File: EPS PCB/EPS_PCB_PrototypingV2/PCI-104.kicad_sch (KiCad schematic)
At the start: 6 parts, among them J1 Conn_02x26_Row_Letter_First, J2 Conn_02x26_Row_Letter_First

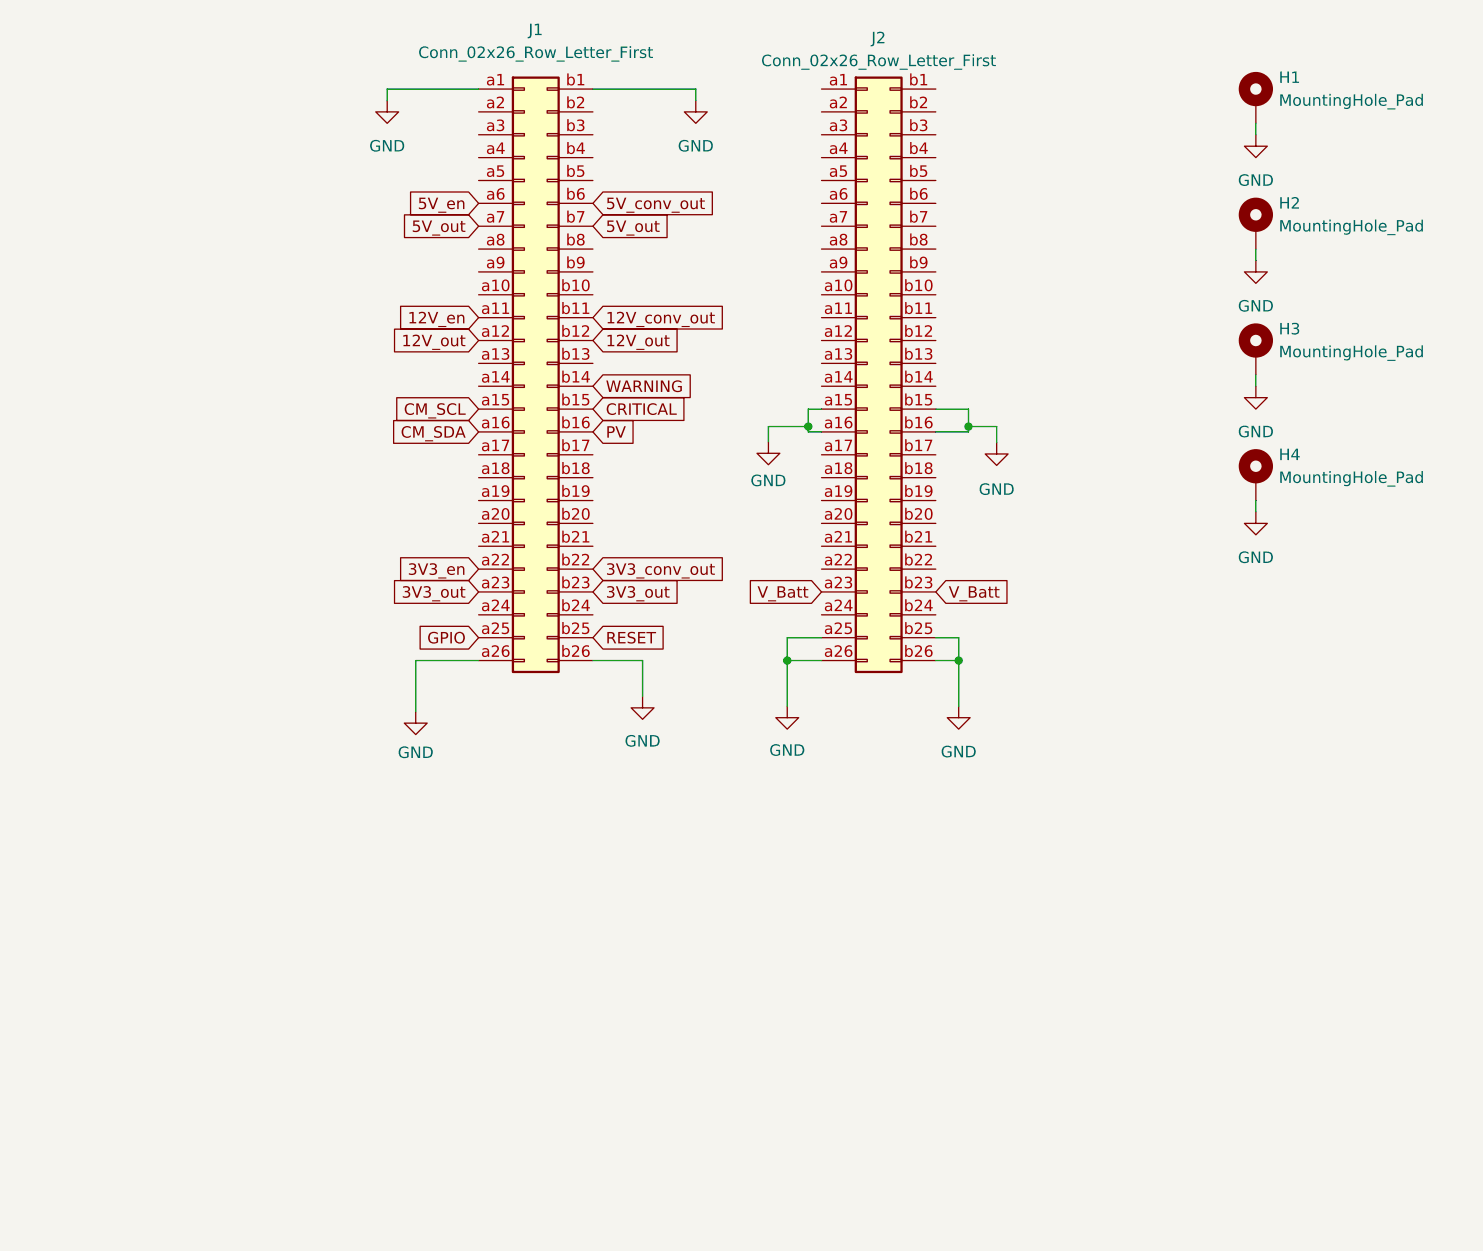
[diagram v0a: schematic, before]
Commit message: EPS PCB Ready for Order
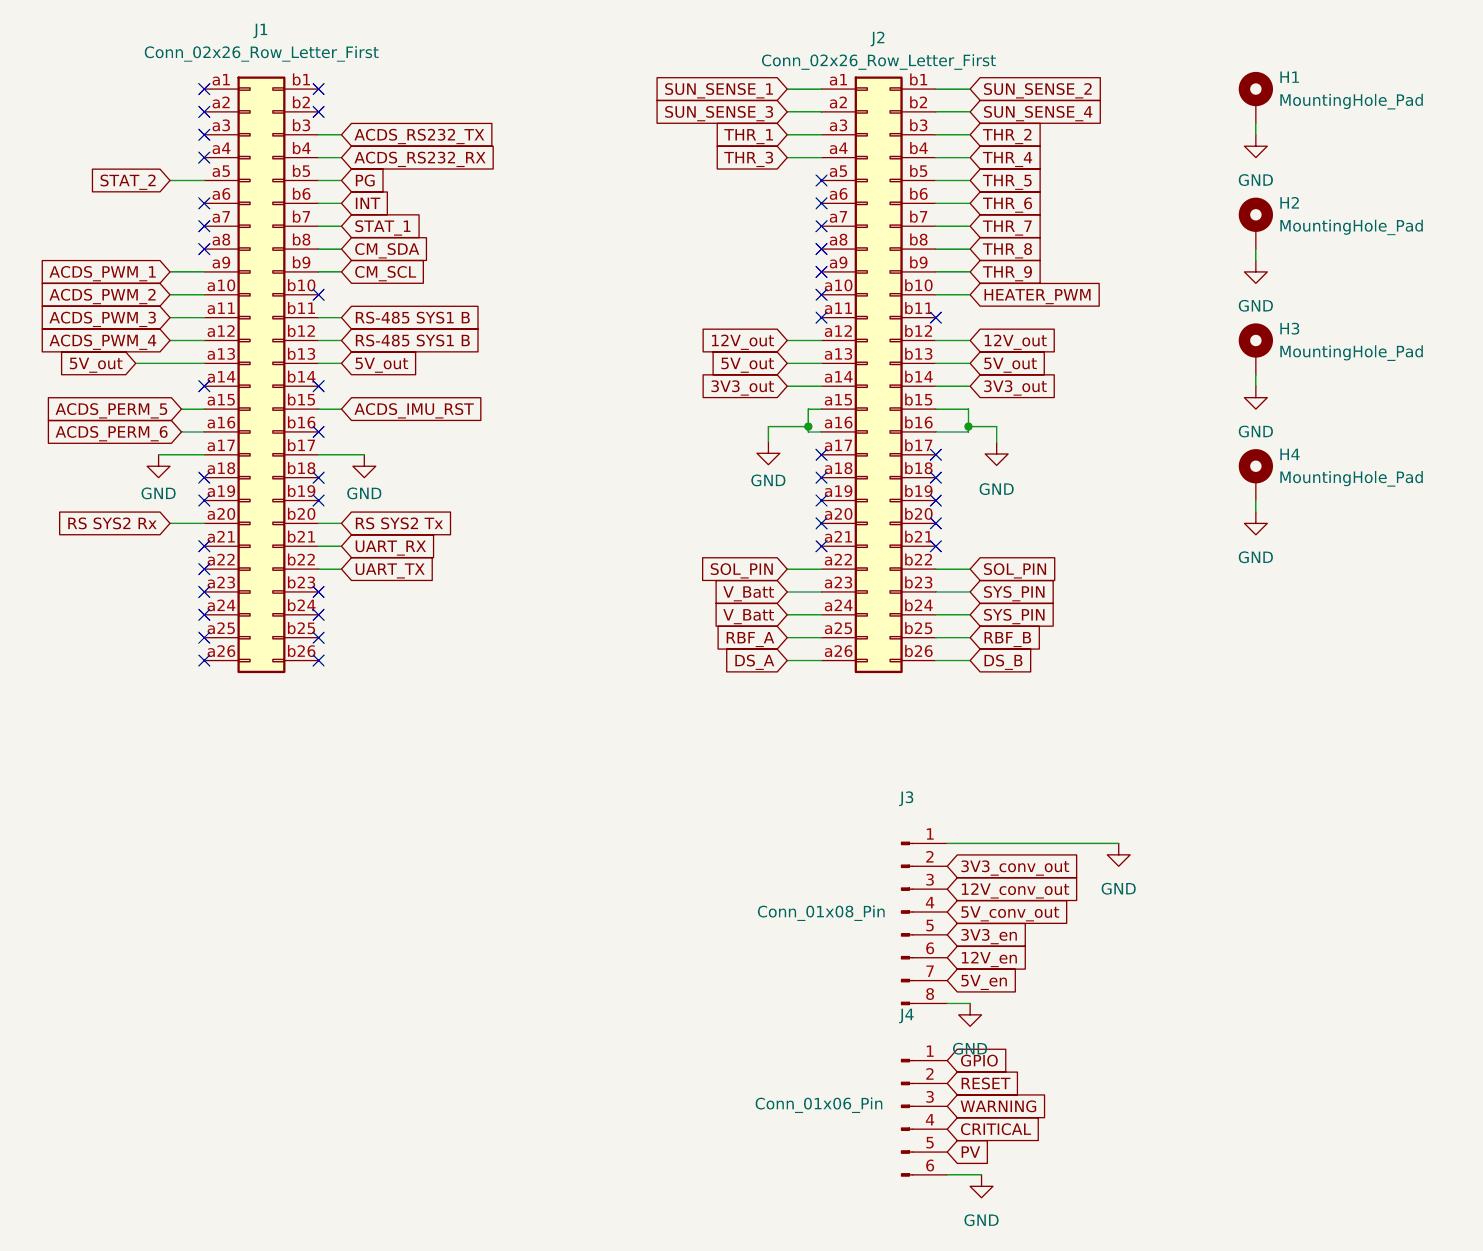
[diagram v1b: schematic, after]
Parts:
- added J3: Conn_01x08_Pin, Connector_PinHeader_2.54mm:PinHeader_1x08_P2.54mm_Vertical, symbol Connector:Conn_01x08_Pin
- added J4: Conn_01x06_Pin, Connector_PinHeader_2.54mm:PinHeader_1x06_P2.54mm_Horizontal, symbol Connector:Conn_01x06_Pin
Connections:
- net 12V_conv_out: now also J3.3 (Pin_3); no longer J1.b11 (Pin_b11)
- net 12V_en: now also J3.6 (Pin_6); no longer J1.a11 (Pin_a11)
- net 12V_out: now also J2.a12 (Pin_a12), J2.b12 (Pin_b12); no longer J1.a12 (Pin_a12), J1.b12 (Pin_b12)
- net 3V3_conv_out: now also J3.2 (Pin_2); no longer J1.b22 (Pin_b22)
- net 3V3_en: now also J3.5 (Pin_5); no longer J1.a22 (Pin_a22)
- net 3V3_out: now also J2.a14 (Pin_a14), J2.b14 (Pin_b14); no longer J1.a23 (Pin_a23), J1.b23 (Pin_b23)
- net 5V_conv_out: now also J3.4 (Pin_4); no longer J1.b6 (Pin_b6)
- net 5V_en: now also J3.7 (Pin_7); no longer J1.a6 (Pin_a6)
- net 5V_out: now also J1.a13 (Pin_a13), J1.b13 (Pin_b13), J2.a13 (Pin_a13), J2.b13 (Pin_b13); no longer J1.a7 (Pin_a7), J1.b7 (Pin_b7)
- net CM_SCL: now also J1.b9 (Pin_b9); no longer J1.a15 (Pin_a15)
- net CM_SDA: now also J1.b8 (Pin_b8); no longer J1.a16 (Pin_a16)
- net CRITICAL: now also J4.4 (Pin_4); no longer J1.b15 (Pin_b15)
- net GND: now also J1.a17 (Pin_a17), J1.b17 (Pin_b17), J3.1 (Pin_1), J3.8 (Pin_8), J4.6 (Pin_6); no longer J1.a1 (Pin_a1), J1.a26 (Pin_a26), J1.b1 (Pin_b1), J1.b26 (Pin_b26), J2.a25 (Pin_a25), J2.a26 (Pin_a26), J2.b25 (Pin_b25), J2.b26 (Pin_b26)
- net GPIO: now also J4.1 (Pin_1); no longer J1.a25 (Pin_a25)
- net PV: now also J4.5 (Pin_5); no longer J1.b16 (Pin_b16)
- net RESET: now also J4.2 (Pin_2); no longer J1.b25 (Pin_b25)
- net V_Batt: now also J2.a24 (Pin_a24); no longer J2.b23 (Pin_b23)
- net WARNING: now also J4.3 (Pin_3); no longer J1.b14 (Pin_b14)
- net ACDS_PWM_2: now reaches J1.a10 (Pin_a10)
- net RS SYS2 Rx: now reaches J1.a20 (Pin_a20)
- net STAT_2: now reaches J1.a5 (Pin_a5)
- net ACDS_PWM_1: now reaches J1.a9 (Pin_a9)
- net RS SYS2 Tx: now reaches J1.b20 (Pin_b20)
- net UART_RX: now reaches J1.b21 (Pin_b21)
- net ACDS_RS232_TX: now reaches J1.b3 (Pin_b3)
- net ACDS_RS232_RX: now reaches J1.b4 (Pin_b4)
- net PG: now reaches J1.b5 (Pin_b5)
- net SUN_SENSE_1: now reaches J2.a1 (Pin_a1)
- net SUN_SENSE_3: now reaches J2.a2 (Pin_a2)
- net SOL_PIN: now reaches J2.a22 (Pin_a22)
- net SOL_PIN: now also J2.b22 (Pin_b22)
- net THR_1: now reaches J2.a3 (Pin_a3)
- net THR_3: now reaches J2.a4 (Pin_a4)
- net SUN_SENSE_2: now reaches J2.b1 (Pin_b1)
- net HEATER_PWM: now reaches J2.b10 (Pin_b10)
- net SUN_SENSE_4: now reaches J2.b2 (Pin_b2)
- net SYS_PIN: now reaches J2.b24 (Pin_b24)
- net SYS_PIN: now also J2.b23 (Pin_b23)
- net THR_2: now reaches J2.b3 (Pin_b3)
- net THR_4: now reaches J2.b4 (Pin_b4)
- net THR_5: now reaches J2.b5 (Pin_b5)
- net THR_6: now reaches J2.b6 (Pin_b6)
- net THR_7: now reaches J2.b7 (Pin_b7)
- net THR_8: now reaches J2.b8 (Pin_b8)
- net THR_9: now reaches J2.b9 (Pin_b9)
- new net ACDS_IMU_RST: J1.b15 (Pin_b15)
- new net ACDS_PERM_5: J1.a15 (Pin_a15)
- new net ACDS_PERM_6: J1.a16 (Pin_a16)
- new net ACDS_PWM_3: J1.a11 (Pin_a11)
- new net ACDS_PWM_4: J1.a12 (Pin_a12)
- new net DS_A: J2.a26 (Pin_a26)
- new net DS_B: J2.b26 (Pin_b26)
- new net INT: J1.b6 (Pin_b6)
- new net RBF_A: J2.a25 (Pin_a25)
- new net RBF_B: J2.b25 (Pin_b25)
- new net RS-485 SYS1 B: J1.b11 (Pin_b11), J1.b12 (Pin_b12)
- new net STAT_1: J1.b7 (Pin_b7)
- new net UART_TX: J1.b22 (Pin_b22)
- no-connect marks 0 -> 45
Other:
- moved on the sheet: J1
